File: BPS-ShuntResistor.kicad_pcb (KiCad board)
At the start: 2 copper layers, 40.1 x 35.1 mm, 18 parts, among them J3 Amp_Conn, SW1 SW_DPST

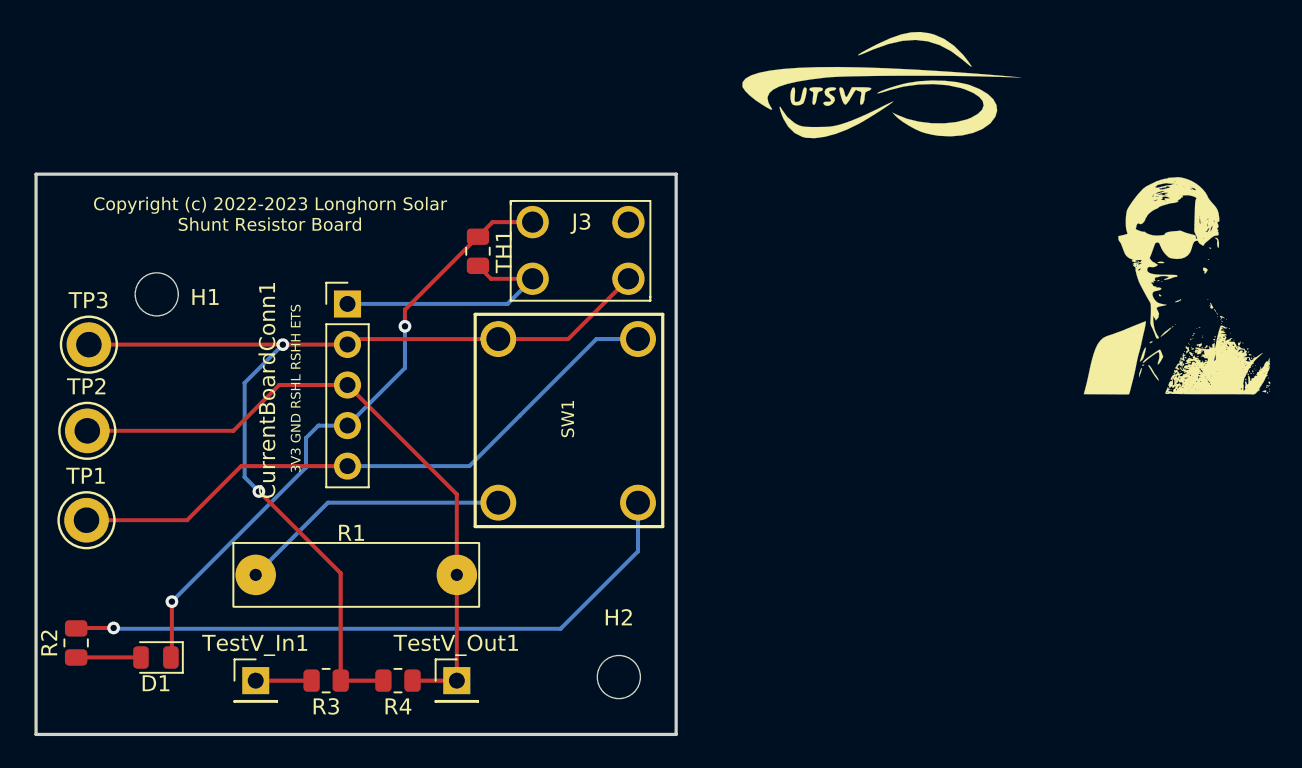
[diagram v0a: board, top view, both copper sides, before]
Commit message: updating custom board parts
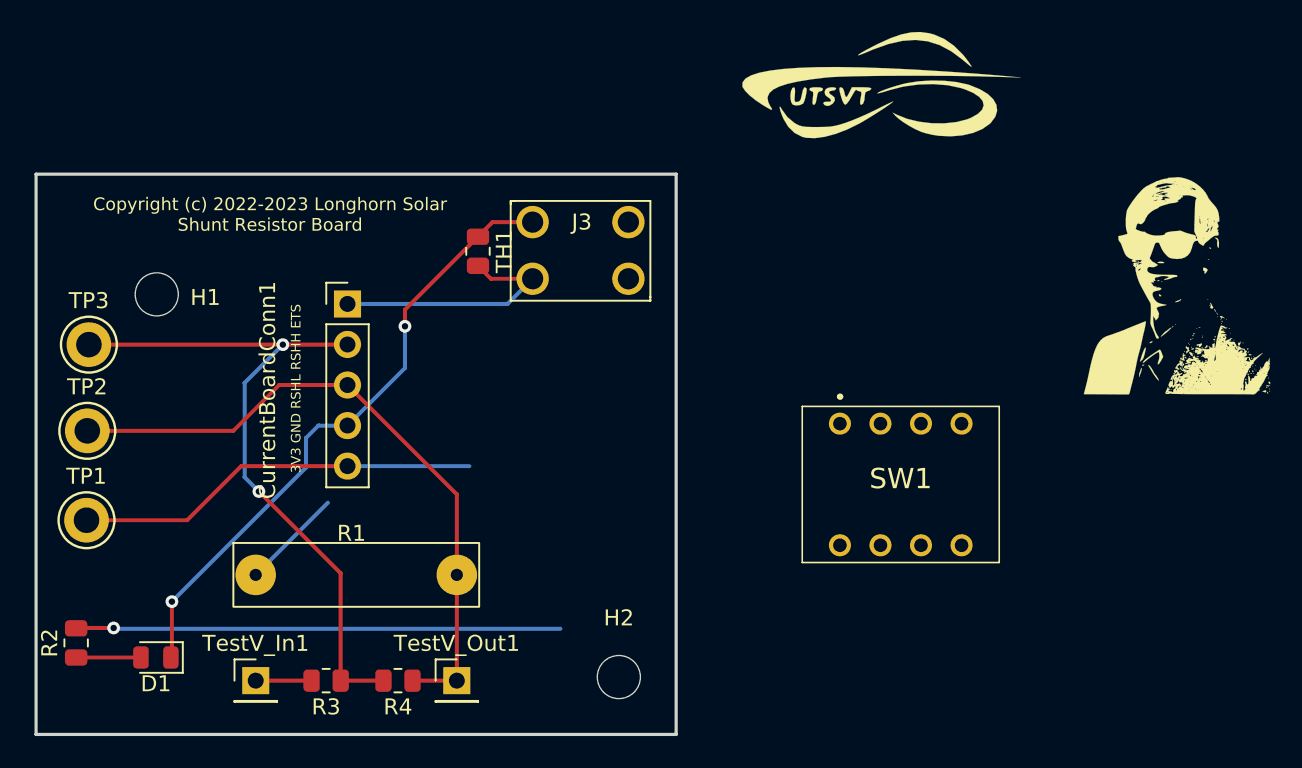
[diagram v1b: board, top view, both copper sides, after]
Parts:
- SW1: footprint UTSVT_Special:SDDJE32700 -> UTSVT_Special:206212
- moved SW1 17.0 mm to (158.8, 93.1), turned to 0 degrees
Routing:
- net RSHH: track 62.7 -> 43.9 mm
- net +3V3: track 39.3 -> 25.4 mm
- net Net-(R1-Pad1): track 17.1 -> 6.40 mm
- net Net-(R2-Pad2): track 40.3 -> 30.4 mm
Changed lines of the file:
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@@
     )
   )
-  (footprint "UTSVT_Special:SDDJE32700" (layer "F.Cu")
-    (at 141.825 92.8 90)
-    (property "Sheetfile" "BPS-ShuntResistor.kicad_sch")
-    (property "Sheetname" "")
-    (attr through_hole)
-    (fp_text reference "SW1" (at 0 0 90) (layer "F.SilkS")
-      (effects (font (size 0.787402 0.787402) (thickness 0.15)))
-    )
-    (fp_text value "SW_DPST" (at 0 0 90) (layer "F.Fab")
-      (effects (font (size 0.787402 0.787402) (thickness 0.15)))
-    )
-    (pad "1" thru_hole circle (at -5.25 -4.375 90) (size 2.25 2.25) (drill 1.5) (layers *.Cu *.Mask)
-      (net 7 "Net-(R1-Pad1)") (pinfunction "1") (pintype "passive"))
-    (pad "2" thru_hole circle (at 5 -4.375 90) (size 2.25 2.25) (drill 1.5) (layers *.Cu *.Mask)
-      (net 3 "RSHH") (pinfunction "2") (pintype "passive"))
-    (pad "3" thru_hole circle (at -5.25 4.375 90) (size 2.25 2.25) (drill 1.5) (layers *.Cu *.Mask)
-      (net 8 "Net-(R2-Pad2)") (pinfunction "3") (pintype "passive"))
-    (pad "4" thru_hole circle (at 5 4.375 90) (size 2.25 2.25) (drill 1.5) (layers *.Cu *.Mask)
-      (net 4 "+3V3") (pinfunction "4") (pintype "passive"))
-  )
   (footprint "Connector_PinHeader_2.54mm:PinHeader_1x01_P2.54mm_Vertical" (layer "F.Cu")
     (at 122.25 109.2)
@@
     (pad "" np_thru_hole circle (at 0 0) (size 2.7 2.7) (drill 2.7) (layers *.Cu *.Mask))
   )
+  (footprint "UTSVT_Special:206212" (layer "F.Cu")
+    (at 158.85 93.1)
+    (descr "206-212-1")
+    (tags "Switch")
+    (property "Sheetfile" "BPS-ShuntResistor.kicad_sch")
+    (property "Sheetname" "")
+    (attr through_hole)
+    (fp_text reference "SW1" (at 3.81 3.455) (layer "F.SilkS")
+      (effects (font (size 1.27 1.27) (thickness 0.254)))
+    )
+    (fp_text value "SW_DPST" (at 3.81 3.455) (layer "F.SilkS") hide
+      (effects (font (size 1.27 1.27) (thickness 0.254)))
+    )
+    (fp_text user "${REFERENCE}" (at 3.81 3.455) (layer "F.Fab")
+      (effects (font (size 1.27 1.27) (thickness 0.254)))
+    )
+    (fp_line (start 0.11 -1.69) (end 0.11 -1.69) (layer "F.SilkS") (width 0.2))
+    (fp_line (start -2.36 8.7) (end -2.36 -1.08) (layer "F.SilkS") (width 0.1))
+    (fp_line (start -0.09 -1.69) (end -0.09 -1.69) (layer "F.SilkS") (width 0.2))
+    (fp_line (start 9.98 8.7) (end -2.36 8.7) (layer "F.SilkS") (width 0.1))
+    (fp_line (start 9.98 -1.08) (end 9.98 8.7) (layer "F.SilkS") (width 0.1))
+    (fp_line (start -2.36 -1.08) (end 9.98 -1.08) (layer "F.SilkS") (width 0.1))
+    (fp_arc (start -0.09 -1.69) (mid 0.01 -1.79) (end 0.11 -1.69) (layer "F.SilkS") (width 0.2))
+    (fp_arc (start 0.11 -1.69) (mid 0.01 -1.59) (end -0.09 -1.69) (layer "F.SilkS") (width 0.2))
+    (fp_line (start -2.86 9.2) (end -2.86 -2.29) (layer "F.CrtYd") (width 0.1))
+    (fp_line (start 10.48 9.2) (end -2.86 9.2) (layer "F.CrtYd") (width 0.1))
+    (fp_line (start 10.48 -2.29) (end 10.48 9.2) (layer "F.CrtYd") (width 0.1))
+    (fp_line (start -2.86 -2.29) (end 10.48 -2.29) (layer "F.CrtYd") (width 0.1))
+    (fp_line (start 9.98 8.7) (end -2.36 8.7) (layer "F.Fab") (width 0.2))
+    (fp_line (start 9.98 -1.08) (end 9.98 8.7) (layer "F.Fab") (width 0.2))
+    (fp_line (start -2.36 8.7) (end -2.36 -1.08) (layer "F.Fab") (width 0.2))
+    (fp_line (start -2.36 -1.08) (end 9.98 -1.08) (layer "F.Fab") (width 0.2))
+    (pad "A1" thru_hole circle locked (at 0 0) (size 1.381 1.381) (drill 0.85) (layers *.Cu *.Mask))
+    (pad "A2" thru_hole circle locked (at 2.54 0) (size 1.381 1.381) (drill 0.85) (layers *.Cu *.Mask))
+    (pad "A3" thru_hole circle locked (at 5.08 0) (size 1.381 1.381) (drill 0.85) (layers *.Cu *.Mask))
+    (pad "A4" thru_hole circle locked (at 7.62 0) (size 1.381 1.381) (drill 0.85) (layers *.Cu *.Mask))
+    (pad "B1" thru_hole circle locked (at 0 7.62) (size 1.381 1.381) (drill 0.85) (layers *.Cu *.Mask))
+    (pad "B2" thru_hole circle locked (at 2.54 7.62) (size 1.381 1.381) (drill 0.85) (layers *.Cu *.Mask))
+    (pad "B3" thru_hole circle locked (at 5.08 7.62) (size 1.381 1.381) (drill 0.85) (layers *.Cu *.Mask))
+    (pad "B4" thru_hole circle locked (at 7.62 7.62) (size 1.381 1.381) (drill 0.85) (layers *.Cu *.Mask))
+    (model "206-212.stp"
+      (offset (xyz 0 0 0))
+      (scale (xyz 1 1 1))
+      (rotate (xyz 0 0 0))
+    )
+  )
   (footprint "TestPoint:TestPoint_Keystone_5005-5009_Compact" (layer "F.Cu")
     (at 111.7 93.55)
@@
     )
   )
-  (gr_rect (start 136 86.25) (end 147.75 99.55) (layer "F.SilkS") (width 0.2) (fill none))
   (gr_rect (start 108.49 77.47) (end 148.59 112.57) (layer "Edge.Cuts") (width 0.2) (fill none))
   (gr_text "Copyright (c) 2022-2023 Longhorn Solar\nShunt Resistor Board" (at 123.15 80) (layer "F.SilkS")
@@
   (segment (start 127.575 109.2) (end 127.575 102.475) (width 0.25) (layer "F.Cu") (net 3))
   (segment (start 128.34 87.8) (end 128 88.14) (width 0.25) (layer "F.Cu") (net 3))
-  (segment (start 137.45 87.8) (end 141.823 87.8) (width 0.25) (layer "F.Cu") (net 3))
   (segment (start 123.95 88.15) (end 127.99 88.15) (width 0.25) (layer "F.Cu") (net 3))
   (segment (start 127.99 88.15) (end 128 88.14) (width 0.25) (layer "F.Cu") (net 3))
   (segment (start 111.8 88.15) (end 123.95 88.15) (width 0.25) (layer "F.Cu") (net 3))
-  (segment (start 137.45 87.8) (end 128.34 87.8) (width 0.25) (layer "F.Cu") (net 3))
   (segment (start 127.575 102.475) (end 122.45 97.35) (width 0.25) (layer "F.Cu") (net 3))
-  (segment (start 141.823 87.8) (end 145.6 84.023) (width 0.25) (layer "F.Cu") (net 3))
   (segment (start 127.575 109.2) (end 130.25 109.2) (width 0.25) (layer "F.Cu") (net 3))
   (via (at 122.45 97.35) (size 0.8) (drill 0.4) (layers "F.Cu" "B.Cu") (net 3))
@@
   (segment (start 121.35 95.75) (end 121.36 95.76) (width 0.25) (layer "F.Cu") (net 4))
   (segment (start 121.36 95.76) (end 128 95.76) (width 0.25) (layer "F.Cu") (net 4))
-  (segment (start 143.6 87.8) (end 146.2 87.8) (width 0.25) (layer "B.Cu") (net 4))
   (segment (start 128 95.76) (end 135.64 95.76) (width 0.25) (layer "B.Cu") (net 4))
-  (segment (start 138.8 92.6) (end 143.6 87.8) (width 0.25) (layer "B.Cu") (net 4))
-  (segment (start 135.64 95.76) (end 138.8 92.6) (width 0.25) (layer "B.Cu") (net 4))
   (segment (start 137.0875 80.475) (end 136.175 81.3875) (width 0.25) (layer "F.Cu") (net 5))
   (segment (start 131.6 85.9625) (end 136.175 81.3875) (width 0.25) (layer "F.Cu") (net 5))
@@
   (segment (start 111 107.75) (end 115.0625 107.75) (width 0.25) (layer "F.Cu") (net 6))
   (segment (start 126.775 98.05) (end 122.25 102.575) (width 0.25) (layer "B.Cu") (net 7))
-  (segment (start 137.45 98.05) (end 126.775 98.05) (width 0.25) (layer "B.Cu") (net 7))
   (segment (start 111.025 105.9) (end 111 105.925) (width 0.25) (layer "F.Cu") (net 8))
   (segment (start 113.35 105.9) (end 111.025 105.9) (width 0.25) (layer "F.Cu") (net 8))
   (via (at 113.35 105.9) (size 0.8) (drill 0.4) (layers "F.Cu" "B.Cu") (net 8))
-  (segment (start 141.35 105.95) (end 146.2 101.1) (width 0.25) (layer "B.Cu") (net 8))
   (segment (start 141.35 105.95) (end 113.4 105.95) (width 0.25) (layer "B.Cu") (net 8))
-  (segment (start 146.2 101.1) (end 146.2 98.05) (width 0.25) (layer "B.Cu") (net 8))
   (segment (start 113.4 105.95) (end 113.35 105.9) (width 0.25) (layer "B.Cu") (net 8))
   (segment (start 122.25 109.2) (end 125.75 109.2) (width 0.25) (layer "F.Cu") (net 9))
